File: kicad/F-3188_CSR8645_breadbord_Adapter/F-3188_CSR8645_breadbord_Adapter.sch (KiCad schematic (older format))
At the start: 13 parts, among them J1 SCJ368R1NUS0B00G, J2 ON, P1 CONN_01X22, P2 CONN_01X21, SW1 RESET, SW2 POWER_ON, U1 F-3188_CSR8645

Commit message: to fcking much changes to commit it separatly, lets go with everything in one commit, git will love me for sure :D
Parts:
- D1, D2: symbol LED -> F-3188_CSR8645_breadbord_Adapter-rescue:LED-RESCUE-F-3188_CSR8645_breadbord_Adapter
- J1: symbol SCJ368R1NUS0B00G -> F-3188_CSR8645_breadbord_Adapter-rescue:SCJ368R1NUS0B00G-RESCUE-F-3188_CSR8645_breadbord_Adapter
- J2: symbol GS2 -> F-3188_CSR8645_breadbord_Adapter-rescue:GS2-RESCUE-F-3188_CSR8645_breadbord_Adapter
- P1: symbol CONN_01X22 -> F-3188_CSR8645_breadbord_Adapter-rescue:CONN_01X22-RESCUE-F-3188_CSR8645_breadbord_Adapter
- P2: symbol CONN_01X21 -> F-3188_CSR8645_breadbord_Adapter-rescue:CONN_01X21-RESCUE-F-3188_CSR8645_breadbord_Adapter
- R1, R2, R3, R4: symbol R -> F-3188_CSR8645_breadbord_Adapter-rescue:R-RESCUE-F-3188_CSR8645_breadbord_Adapter
- SW1, SW2: symbol SW_Push -> F-3188_CSR8645_breadbord_Adapter-rescue:SW_Push-RESCUE-F-3188_CSR8645_breadbord_Adapter
- U1: symbol F-3188_CSR8645 -> F-3188_CSR8645:F-3188_CSR8645
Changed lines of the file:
@@
-EESchema Schematic File Version 2
-LIBS:power
-LIBS:device
-LIBS:transistors
-LIBS:conn
-LIBS:linear
-LIBS:regul
-LIBS:74xx
-LIBS:cmos4000
-LIBS:adc-dac
-LIBS:memory
-LIBS:xilinx
-LIBS:microcontrollers
-LIBS:dsp
-LIBS:microchip
-LIBS:analog_switches
-LIBS:motorola
-LIBS:texas
-LIBS:intel
-LIBS:audio
-LIBS:interface
-LIBS:digital-audio
-LIBS:philips
-LIBS:display
-LIBS:cypress
-LIBS:siliconi
-LIBS:opto
-LIBS:atmel
-LIBS:contrib
-LIBS:valves
-LIBS:F-3188_CSR8645
-LIBS:phonejack
-LIBS:switches
+EESchema Schematic File Version 4
 LIBS:F-3188_CSR8645_breadbord_Adapter-cache
 EELAYER 26 0
@@
 $EndDescr
 $Comp
-L F-3188_CSR8645 U1
+L F-3188_CSR8645:F-3188_CSR8645 U1
 U 1 1 56E97AB3
 P 6000 4150
@@
 $EndComp
 $Comp
-L CONN_01X21 P2
+L F-3188_CSR8645_breadbord_Adapter-rescue:CONN_01X21-RESCUE-F-3188_CSR8645_breadbord_Adapter P2
 U 1 1 56E97AFF
 P 7400 3600
@@
 $EndComp
 $Comp
-L CONN_01X22 P1
+L F-3188_CSR8645_breadbord_Adapter-rescue:CONN_01X22-RESCUE-F-3188_CSR8645_breadbord_Adapter P1
 U 1 1 56E97BD5
 P 4150 3650
@@
 $EndComp
 $Comp
-L SCJ368R1NUS0B00G J1
+L F-3188_CSR8645_breadbord_Adapter-rescue:SCJ368R1NUS0B00G-RESCUE-F-3188_CSR8645_breadbord_Adapter J1
 U 1 1 56E988D9
 P 9150 5500
@@
 $EndComp
 $Comp
-L LED D2
+L F-3188_CSR8645_breadbord_Adapter-rescue:LED-RESCUE-F-3188_CSR8645_breadbord_Adapter D2
 U 1 1 59A3B48E
 P 2650 4900
@@
 $EndComp
 $Comp
-L R R4
+L F-3188_CSR8645_breadbord_Adapter-rescue:R-RESCUE-F-3188_CSR8645_breadbord_Adapter R4
 U 1 1 59A3B572
 P 2150 4900
@@
 $EndComp
 $Comp
-L R R3
+L F-3188_CSR8645_breadbord_Adapter-rescue:R-RESCUE-F-3188_CSR8645_breadbord_Adapter R3
 U 1 1 59A3B74C
 P 2150 4550
@@
 $EndComp
 $Comp
-L LED D1
+L F-3188_CSR8645_breadbord_Adapter-rescue:LED-RESCUE-F-3188_CSR8645_breadbord_Adapter D1
 U 1 1 59A3B7BD
 P 2650 4550
@@
 	8900 5350 8750 5350
 Wire Wire Line
-	8750 5350 8750 5450
+	8750 5350 8750 5400
 Wire Wire Line
 	8750 5650 8900 5650
 Wire Wire Line
-	8750 5550 8750 5650
+	8750 5550 8750 5600
 Wire Wire Line
 	8750 5600 7900 5600
@@
 LED0
 $Comp
-L SW_Push SW1
+L F-3188_CSR8645_breadbord_Adapter-rescue:SW_Push-RESCUE-F-3188_CSR8645_breadbord_Adapter SW1
 U 1 1 59A3B90C
 P 2600 5450
@@
 $EndComp
 $Comp
-L SW_Push SW2
+L F-3188_CSR8645_breadbord_Adapter-rescue:SW_Push-RESCUE-F-3188_CSR8645_breadbord_Adapter SW2
 U 1 1 59A3B9B6
 P 2600 5900
@@
 RST#
 $Comp
-L R R2
+L F-3188_CSR8645_breadbord_Adapter-rescue:R-RESCUE-F-3188_CSR8645_breadbord_Adapter R2
 U 1 1 59A3BD2D
 P 1950 5900
@@
 $EndComp
 $Comp
-L R R1
+L F-3188_CSR8645_breadbord_Adapter-rescue:R-RESCUE-F-3188_CSR8645_breadbord_Adapter R1
 U 1 1 59A3BDA7
 P 1950 5450
@@
 	2100 5450 2400 5450
 Wire Wire Line
-	2400 5900 2100 5900
-Wire Wire Line
-	2800 5900 3450 5900
+	2400 5900 2250 5900
+Wire Wire Line
+	2800 5900 2900 5900
 Wire Wire Line
 	2800 5450 3450 5450
@@
 BAT
 $Comp
-L GS2 J2
+L F-3188_CSR8645_breadbord_Adapter-rescue:GS2-RESCUE-F-3188_CSR8645_breadbord_Adapter J2
 U 1 1 59A3C964
 P 2600 6250
@@
 	8750 5550 8900 5550
 Connection ~ 8750 5600
+Wire Wire Line
+	2900 5900 3450 5900
+Wire Wire Line
+	2250 5900 2100 5900
+Wire Wire Line
+	8750 5400 8750 5450
+Wire Wire Line
+	8750 5600 8750 5650
 $EndSCHEMATC

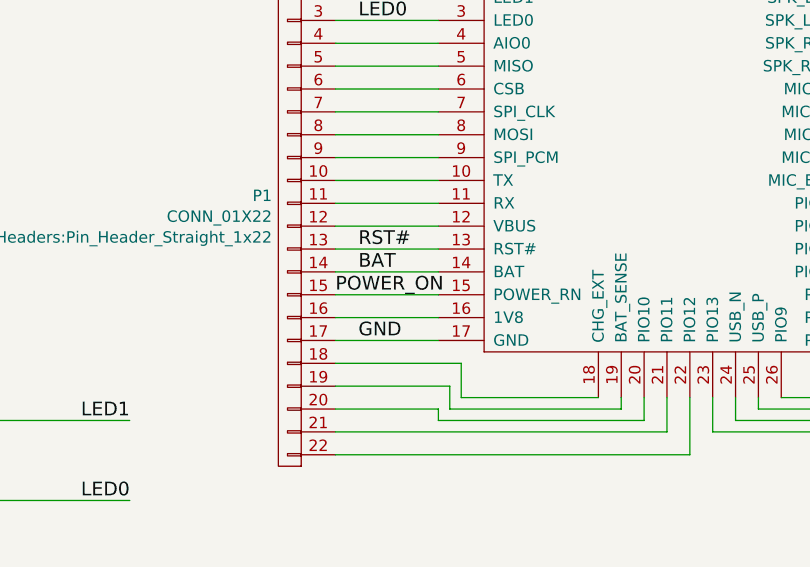
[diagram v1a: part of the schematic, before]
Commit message: new version
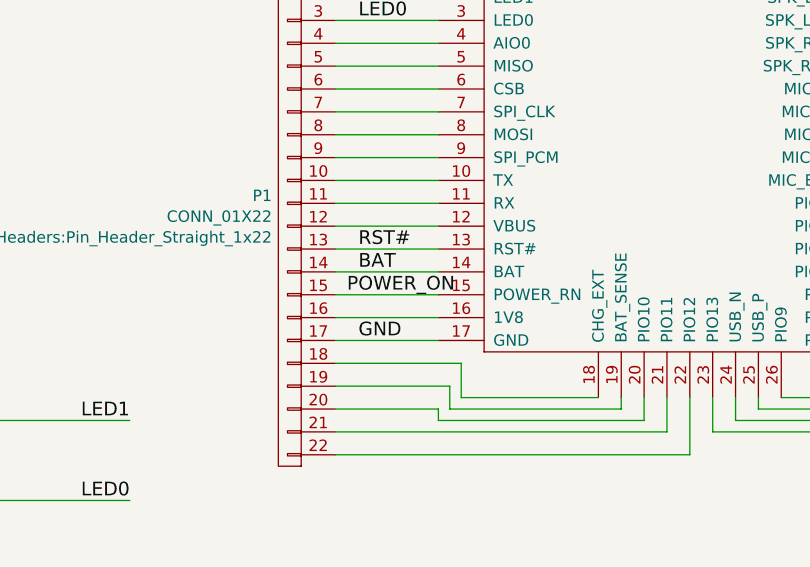
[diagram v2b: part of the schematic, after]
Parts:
- J2: footprint Connectors:GS2 -> Jumper:SolderJumper-2_P1.3mm_Open_RoundedPad1.0x1.5mm
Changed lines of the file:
@@
 F 0 "J2" V 2395 6250 50  0000 C CNN
 F 1 "ON" V 2486 6250 50  0000 C CNN
-F 2 "Connectors:GS2" V 2674 6250 50  0001 C CNN
+F 2 "Jumper:SolderJumper-2_P1.3mm_Open_RoundedPad1.0x1.5mm" V 2674 6250 50  0001 C CNN
 F 3 "" H 2600 6250 50  0001 C CNN
 	1    2600 6250
@@
 	2250 6250 2400 6250
 Connection ~ 2250 5900
-Text Label 4350 4000 0    60   ~ 0
+Text Label 4400 4000 0    60   ~ 0
 POWER_ON
 Wire Wire Line
